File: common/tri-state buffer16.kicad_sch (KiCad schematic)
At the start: 6 parts, among them IC1 SN74AHCT16245DGGR

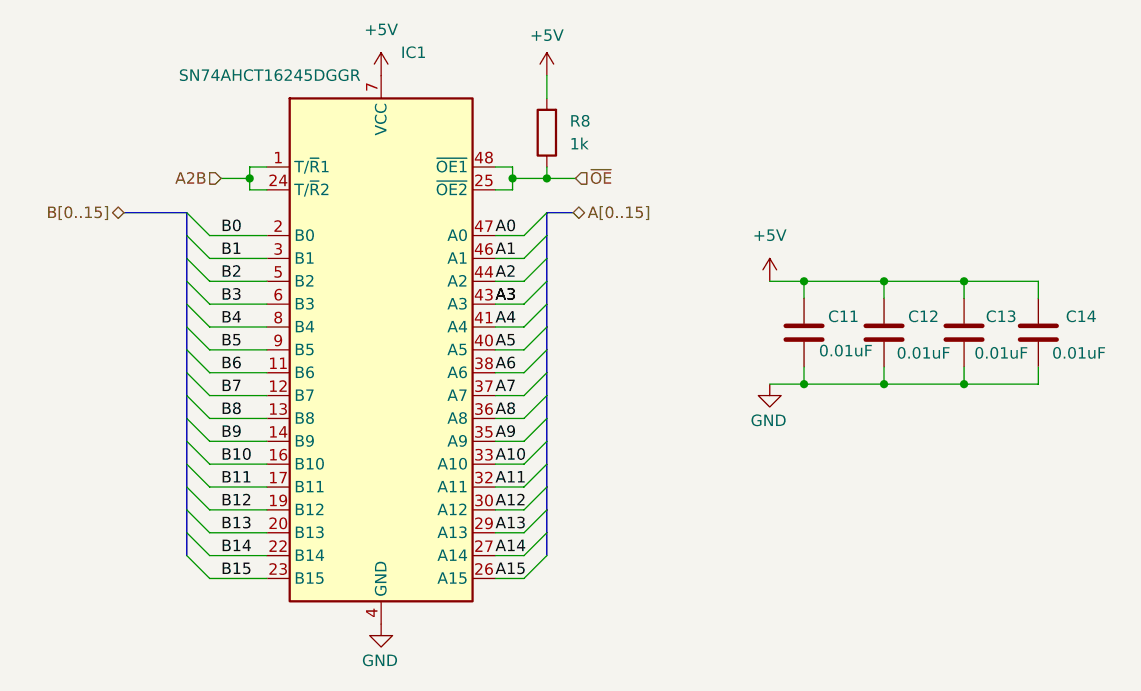
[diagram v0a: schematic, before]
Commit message: Memory Controller- Initial setup
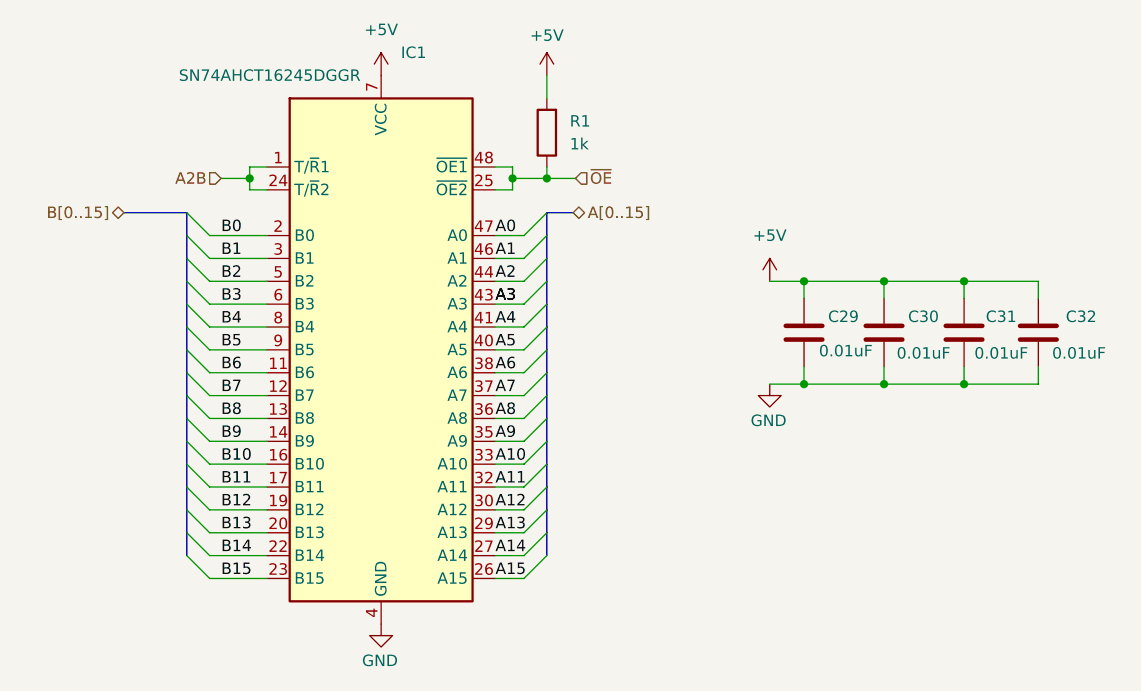
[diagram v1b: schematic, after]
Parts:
- renumbered C11 to C29, C12 to C30, C13 to C31, C14 to C32, R8 to R1
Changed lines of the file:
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@@
 		(on_board yes)
 		(dnp no)
-		(property "Reference" "#PWR052"
+		(property "Reference" "#PWR0102"
 			(at 56.515 106.045 0)
 			(effects
@@
 		(dnp no)
 		(fields_autoplaced yes)
-		(property "Reference" "#PWR048"
+		(property "Reference" "#PWR0103"
 			(at 56.515 42.545 0)
 			(effects
@@
 		(on_board yes)
 		(dnp no)
-		(property "Reference" "#PWR028"
+		(property "Reference" "#PWR0101"
 			(at 99.695 79.375 0)
 			(effects
@@
 		(on_board yes)
 		(dnp no)
-		(property "Reference" "C14"
+		(property "Reference" "C32"
 			(at 132.588 65.532 0)
 			(effects
@@
 		(on_board yes)
 		(dnp no)
-		(property "Reference" "C11"
+		(property "Reference" "C29"
 			(at 106.172 65.532 0)
 			(effects
@@
 		(dnp no)
 		(fields_autoplaced yes)
-		(property "Reference" "#PWR044"
+		(property "Reference" "#PWR0104"
 			(at 74.93 42.545 0)
 			(effects
@@
 		(on_board yes)
 		(dnp no)
-		(property "Reference" "C13"
+		(property "Reference" "C31"
 			(at 123.698 65.532 0)
 			(effects
@@
 		(dnp no)
 		(fields_autoplaced yes)
-		(property "Reference" "#PWR024"
+		(property "Reference" "#PWR0105"
 			(at 99.695 65.405 0)
 			(effects
@@
 		(on_board yes)
 		(dnp no)
-		(property "Reference" "C12"
+		(property "Reference" "C30"
 			(at 115.062 65.532 0)
 			(effects
@@
 		(dnp no)
 		(fields_autoplaced yes)
-		(property "Reference" "R8"
+		(property "Reference" "R1"
 			(at 77.47 43.8149 0)
 			(effects
